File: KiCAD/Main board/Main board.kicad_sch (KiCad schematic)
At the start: 23 parts, among them J1 Conn_01x03, J10 Conn_01x03, J11 Conn_01x03, J12 Conn_01x03, J13 Conn_01x02, J14 Conn_01x02, J15 Conn_01x02, J2 Conn_01x03, J3 Conn_01x02, J4 Conn_01x02, J5 Conn_01x03, J6 Conn_01x02, J7 Conn_01x03, J8 Conn_01x02, J9 Conn_01x03

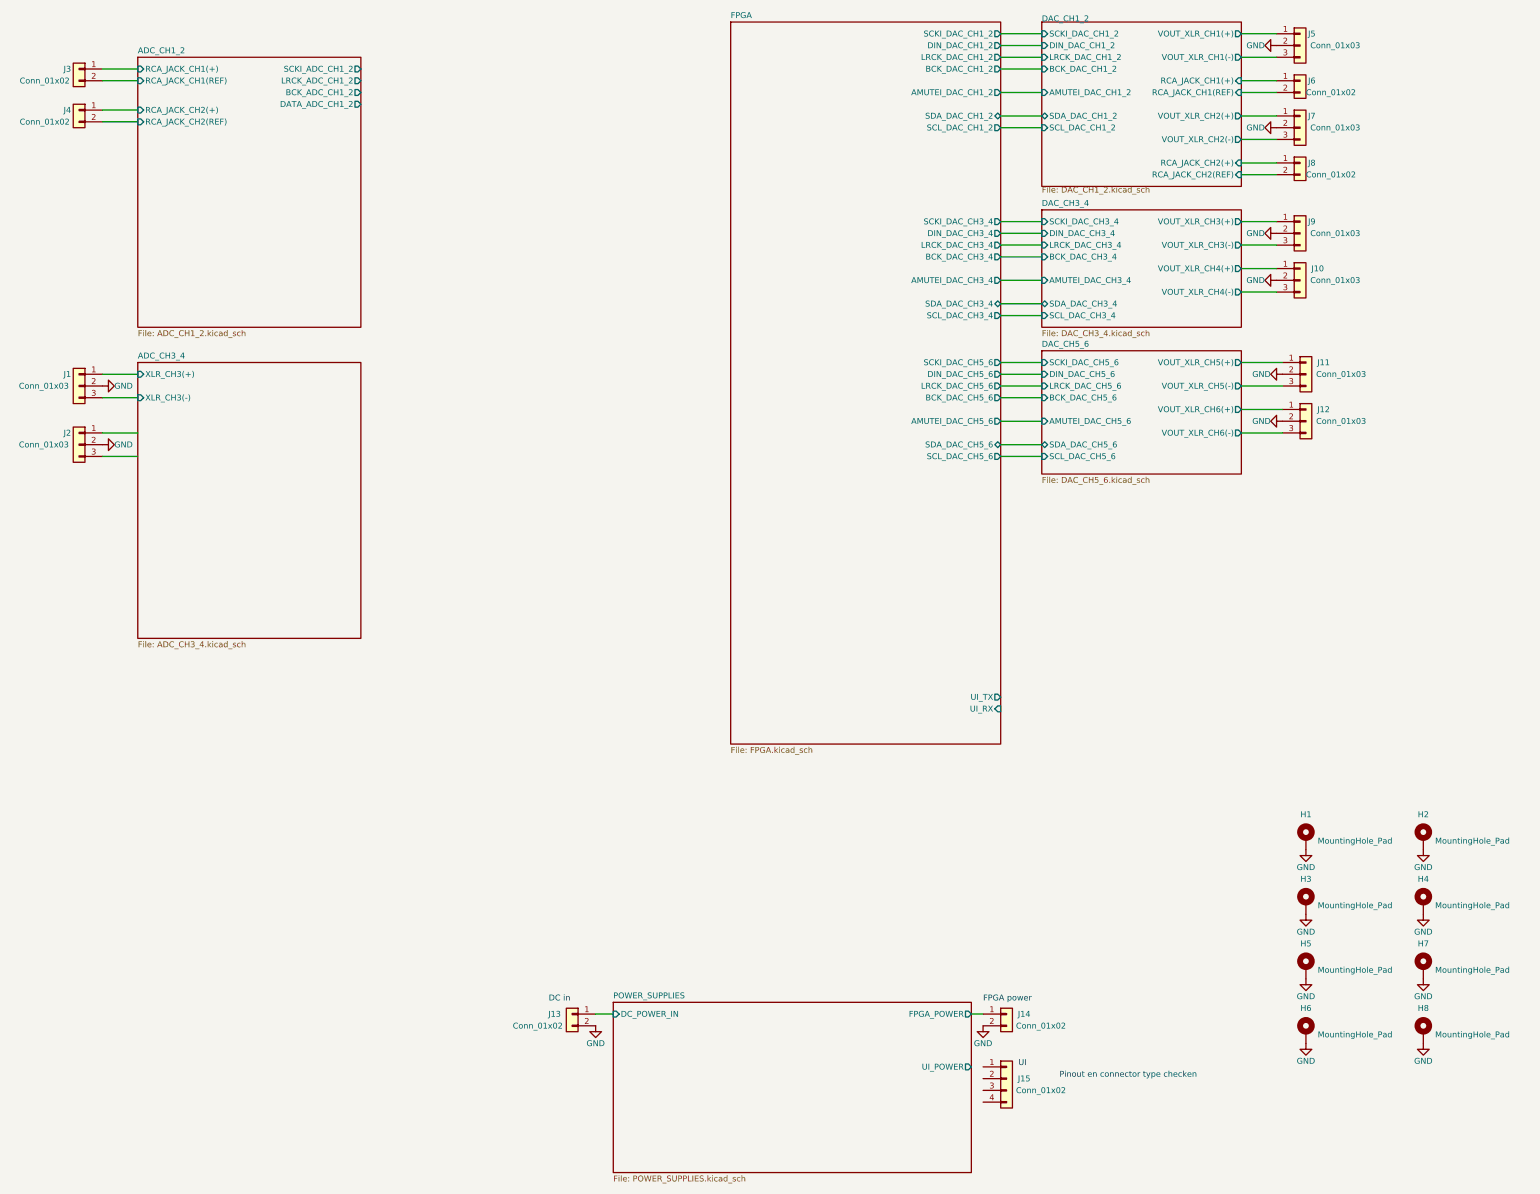
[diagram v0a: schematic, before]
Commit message: Worked on main board design
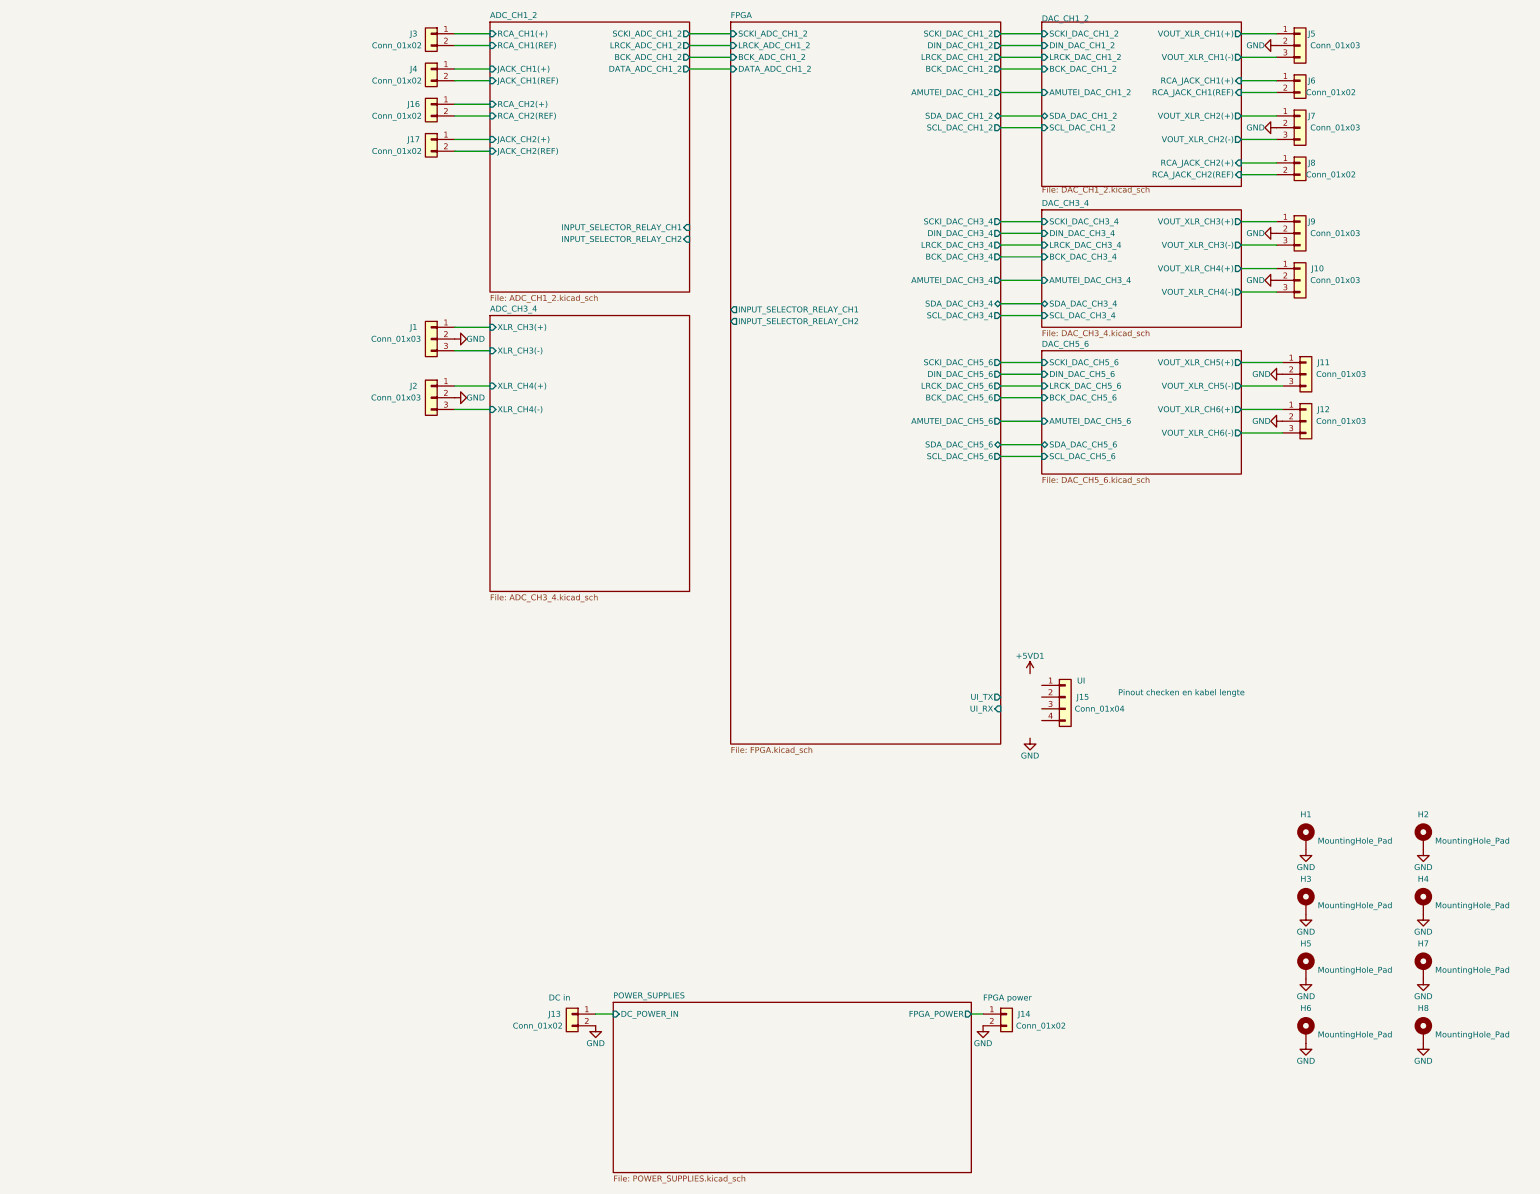
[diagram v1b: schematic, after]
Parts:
- added J16, J17: Conn_01x02, Connector_JST:JST_PH_B2B-PH-K_1x02_P2.00mm_Vertical, symbol Connector_Generic:Conn_01x02
- J15: value Conn_01x02 -> Conn_01x04; footprint Connector_Phoenix_MC:PhoenixContact_MCV_1,5_2-G-3.5_1x02_P3.50mm_Vertical -> Connector_PinHeader_2.54mm:PinHeader_1x04_P2.54mm_Vertical
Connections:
- net ADC_CH3_4/XLR_CH4(+): now reaches J2.1 (Pin_1)
- net ADC_CH3_4/XLR_CH4(-): now reaches J2.3 (Pin_3)
- net ADC_CH1_2/RCA_JACK_CH1(+) renamed ADC_CH1_2/RCA_CH1(+)
- net ADC_CH1_2/RCA_JACK_CH1(REF) renamed ADC_CH1_2/RCA_CH1(REF)
- net ADC_CH1_2/RCA_JACK_CH2(+) renamed ADC_CH1_2/JACK_CH1(+)
- net ADC_CH1_2/RCA_JACK_CH2(REF) renamed ADC_CH1_2/JACK_CH1(REF)
- new net ADC_CH1_2/JACK_CH2(+): J17.1 (Pin_1)
- new net ADC_CH1_2/JACK_CH2(REF): J17.2 (Pin_2)
- new net ADC_CH1_2/RCA_CH2(+): J16.1 (Pin_1)
- new net ADC_CH1_2/RCA_CH2(REF): J16.2 (Pin_2)
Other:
- sheet ADC_CH1_2 ports: added INPUT_SELECTOR_RELAY_CH1, INPUT_SELECTOR_RELAY_CH2, JACK_CH1(+), JACK_CH1(REF), JACK_CH2(+), JACK_CH2(REF), RCA_CH1(+), RCA_CH1(REF), RCA_CH2(+), RCA_CH2(REF); removed RCA_JACK_CH1(+), RCA_JACK_CH1(REF), RCA_JACK_CH2(+), RCA_JACK_CH2(REF)
- sheet ADC_CH3_4 ports: added XLR_CH4(+), XLR_CH4(-); removed none
- sheet FPGA ports: added BCK_ADC_CH1_2, DATA_ADC_CH1_2, INPUT_SELECTOR_RELAY_CH1, INPUT_SELECTOR_RELAY_CH2, LRCK_ADC_CH1_2, SCKI_ADC_CH1_2; removed none
- sheet POWER_SUPPLIES ports: added none; removed UI_POWER
- note added: "Pinout checken en kabel lengte"
- note removed: "Pinout en connector type checken"
- moved on the sheet: J1, J15, J2, J3, J4

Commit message: Worked on main board
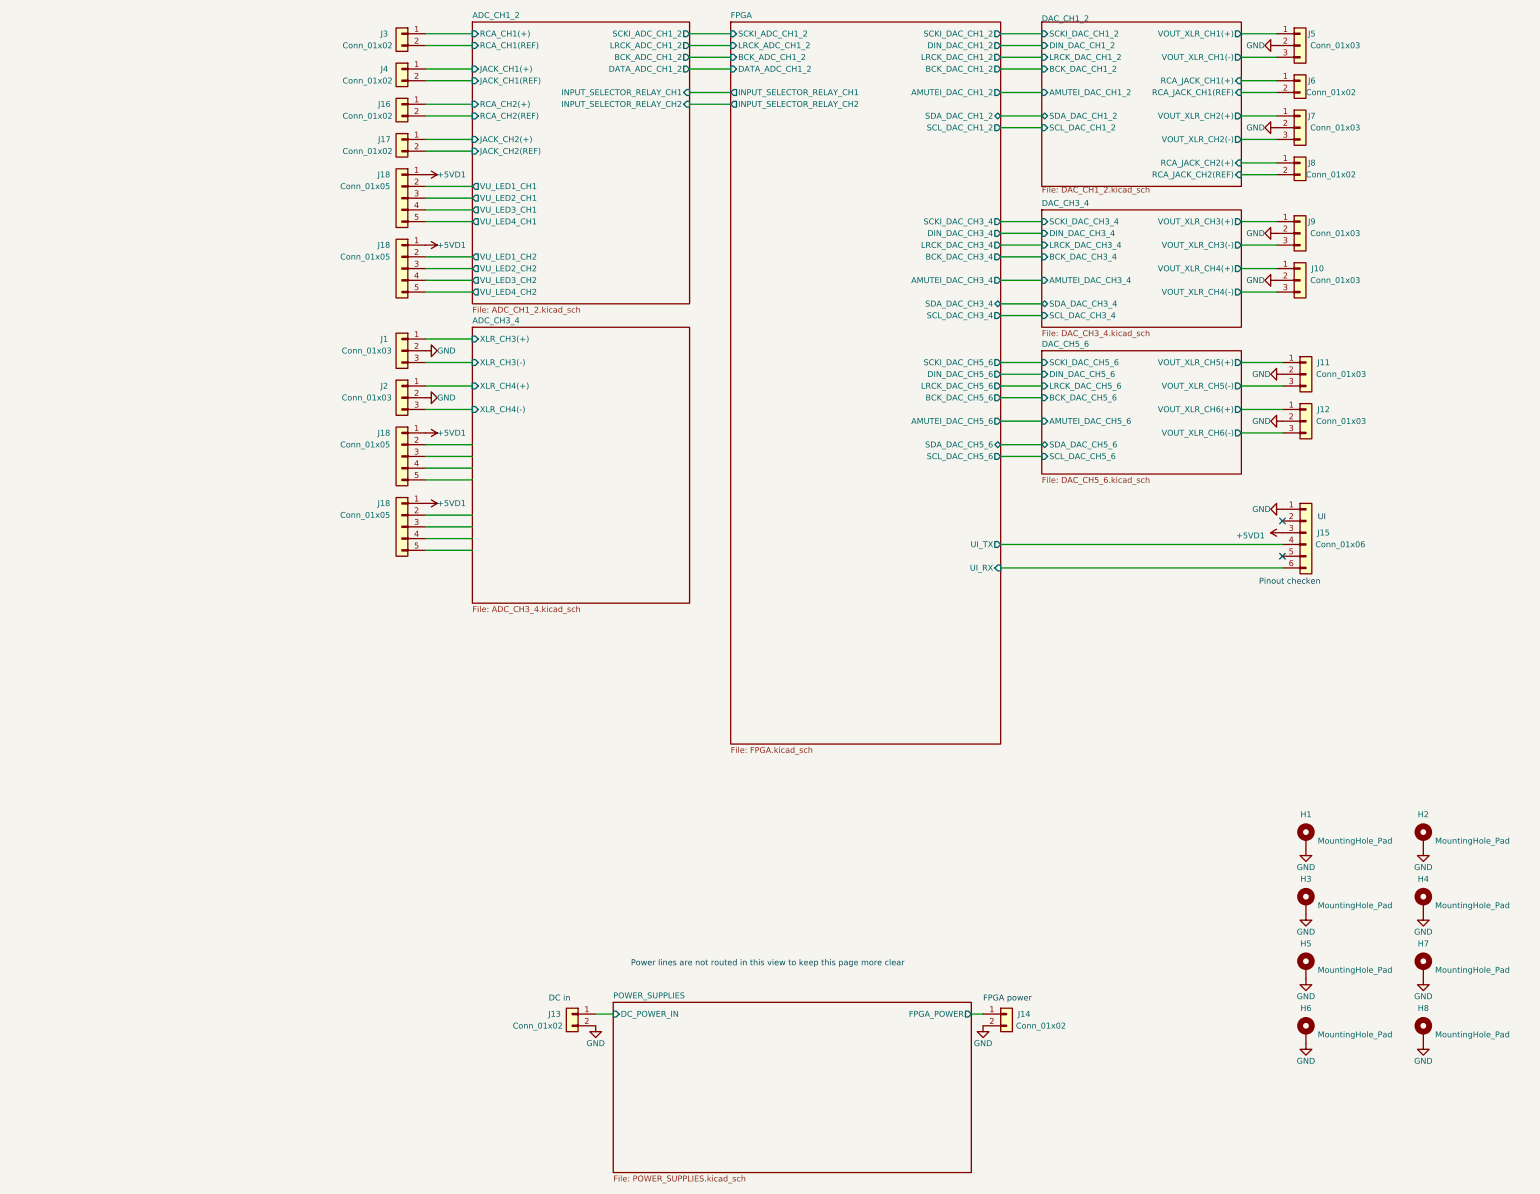
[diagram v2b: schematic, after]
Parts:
- added J18 (x4): Conn_01x05, Connector_JST:JST_XH_B5B-XH-A_1x05_P2.50mm_Vertical, symbol Connector_Generic:Conn_01x05
- J15: value Conn_01x04 -> Conn_01x06; footprint Connector_PinHeader_2.54mm:PinHeader_1x04_P2.54mm_Vertical -> Connector_JST:JST_PH_B6B-PH-K_1x06_P2.00mm_Vertical; symbol Connector_Generic:Conn_01x04 -> Connector_Generic:Conn_01x06; Datasheet cable (none) -> https://www.tinytronics.nl/shop/nl/kabels-en-connectoren/ka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
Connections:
- net +5VD1: now also J15.3 (Pin_3), J18.1 (Pin_1), J18.1 (Pin_1), J18.1 (Pin_1), J18.1 (Pin_1)
- net FPGA/UI_RX: now also J15.6 (Pin_6)
- net FPGA/UI_TX: now also J15.4 (Pin_4)
- net GND: now also J15.1 (Pin_1)
- new net ADC_CH1_2/VU_LED1_CH1: J18.2 (Pin_2)
- new net ADC_CH1_2/VU_LED1_CH2: J18.2 (Pin_2)
- new net ADC_CH1_2/VU_LED2_CH1: J18.3 (Pin_3)
- new net ADC_CH1_2/VU_LED2_CH2: J18.3 (Pin_3)
- new net ADC_CH1_2/VU_LED3_CH1: J18.4 (Pin_4)
- new net ADC_CH1_2/VU_LED3_CH2: J18.4 (Pin_4)
- new net ADC_CH1_2/VU_LED4_CH1: J18.5 (Pin_5)
- new net ADC_CH1_2/VU_LED4_CH2: J18.5 (Pin_5)
- no-connect marks 0 -> 2
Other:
- sheet ADC_CH1_2 ports: added VU_LED1_CH1, VU_LED1_CH2, VU_LED2_CH1, VU_LED2_CH2, VU_LED3_CH1, VU_LED3_CH2, VU_LED4_CH1, VU_LED4_CH2; removed none
- note added: "Pinout checken"
- note added: "Power lines are not routed in this view to keep this page more clear"
- note removed: "Pinout checken en kabel lengte"
- moved on the sheet: J1, J16, J17, J2, J3, J4
